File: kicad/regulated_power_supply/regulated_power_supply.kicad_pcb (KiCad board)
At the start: 2 copper layers, 139.1 x 38.5 mm, 43 parts, among them P1 CONN_01X03, P2 CONN_01X02, Q1 Q_NPN_BCE, SW1 SPST, T1 2N3055, U1 TL072, U2 LM723

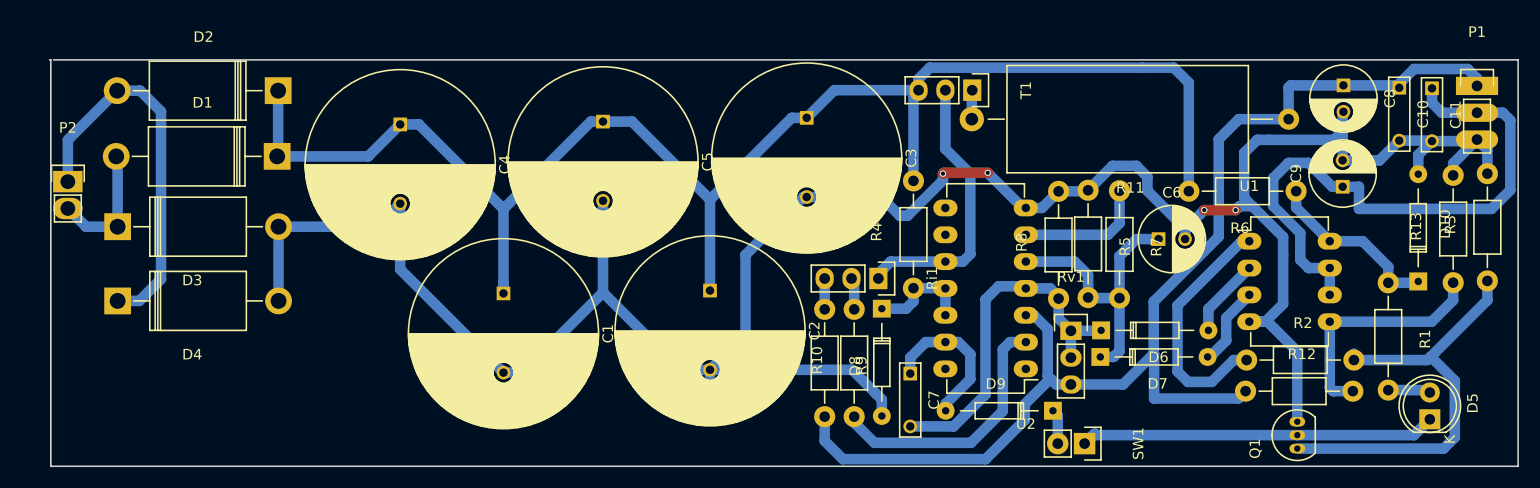
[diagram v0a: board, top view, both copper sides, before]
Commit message: update
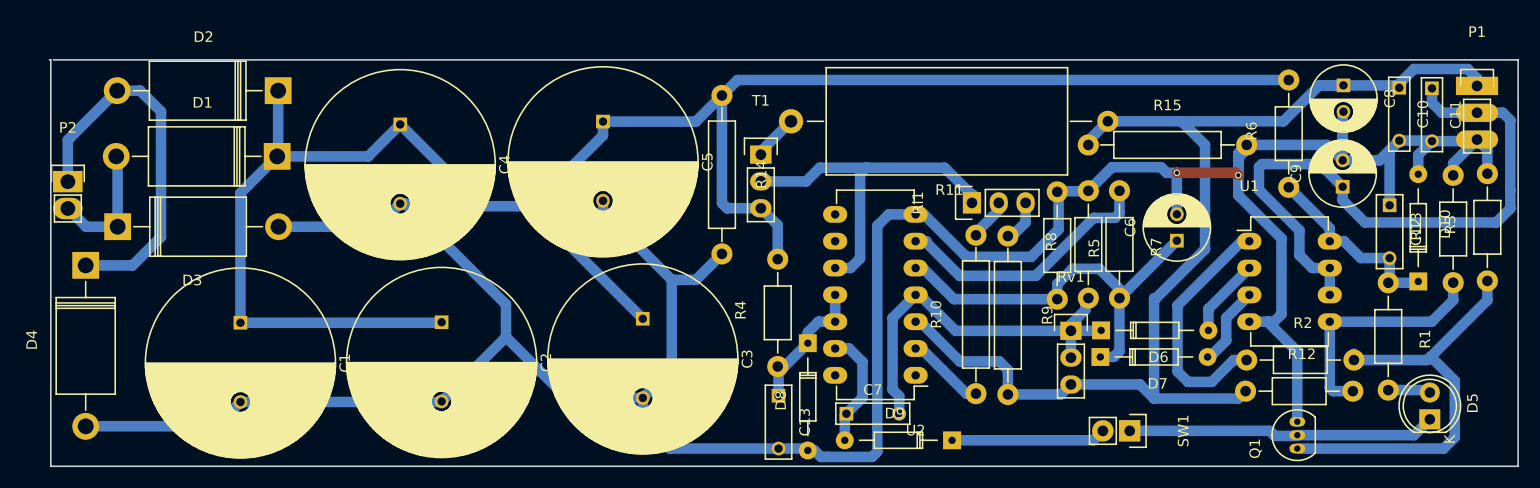
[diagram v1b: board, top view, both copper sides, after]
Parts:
- added C12: 100n, Capacitors_ThroughHole:C_Rect_L7_W2.5_P5, F.Cu at (193.7, 37.3)
- added C13: 100n, Capacitors_ThroughHole:C_Rect_L7_W2.5_P5, F.Cu at (135.8, 55.3)
- added R14: 1K, Resistors_ThroughHole:Resistor_Horizontal_RM15mm, F.Cu at (130.5, 34.4)
- added R15: 1K, Resistors_ThroughHole:Resistor_Horizontal_RM15mm, F.Cu at (172.7, 31.5)
- R10, R9: footprint Resistors_ThroughHole:Resistor_Horizontal_RM10mm -> Resistors_ThroughHole:Resistor_Horizontal_RM15mm
- moved C2 25.6 mm to (103.9, 48.3)
- moved C1 25.1 mm to (84.9, 48.4)
- moved C3 24.6 mm to (123.0, 48.0)
- moved T1 20.9 mm to (134.2, 32.5), turned to 0 degrees
- moved R9 17.9 mm to (157.6, 47.7)
- moved R11 17.1 mm to (152.0, 29.3)
- moved R4 14.8 mm to (135.8, 47.4)
- moved R10 12.4 mm to (154.5, 47.6)
- moved Ri1 11.4 mm to (154.2, 37.0), turned to 90 degrees
- moved U2 10.5 mm to (148.8, 53.4)
- moved D9 9.95 mm to (152.3, 59.5)
- moved D8 7.73 mm to (138.6, 50.3)
- moved C7 7.14 mm to (142.3, 57.0), turned to 0 degrees
- moved R6 6.99 mm to (184.2, 30.5), turned to 90 degrees
- moved D4 4.53 mm to (70.2, 43.0), turned to 270 degrees
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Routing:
- net GND: track 241.3 -> 292.4 mm, vias 4 -> 2
- net /Vin: track 145.9 -> 183.1 mm
- net Net-(R10-Pad1): track 25.7 -> 7.49 mm
- net Net-(R7-Pad1): track 12.4 -> 26.1 mm
- net Net-(C6-Pad1): track 27.1 -> 39.4 mm
- net Net-(D9-Pad1): track 3.30 -> 14.6 mm
- net /Bt1: track 26.4 -> 34.6 mm
- net Net-(D5-Pad1): track 35.0 -> 29.3 mm
- net /Vout: track 115.6 -> 111.1 mm
- net /Vhalf: track 57.4 -> 61.2 mm
- net Net-(C7-Pad1): track 14.6 -> 11.2 mm
- net Net-(C7-Pad2): track 34.4 -> 37.5 mm
- net /V723: track 10.1 -> 13.1 mm
- net Net-(R9-Pad1): track 2.92 -> 4.43 mm
- net Net-(R11-Pad2): track 2.85 -> 4.33 mm
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
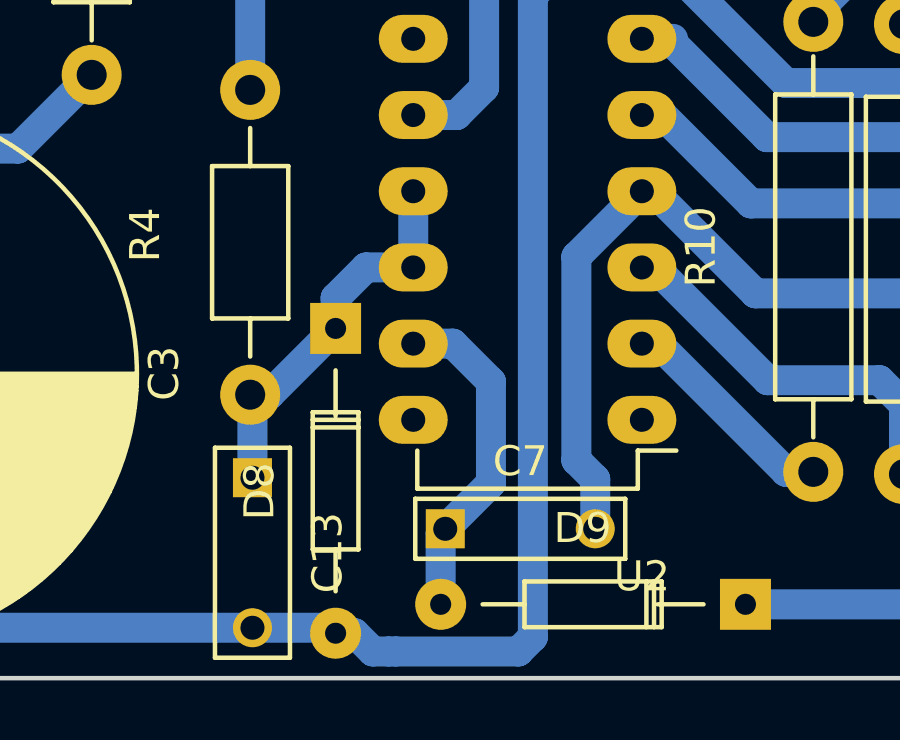
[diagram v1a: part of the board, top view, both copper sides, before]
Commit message: updates
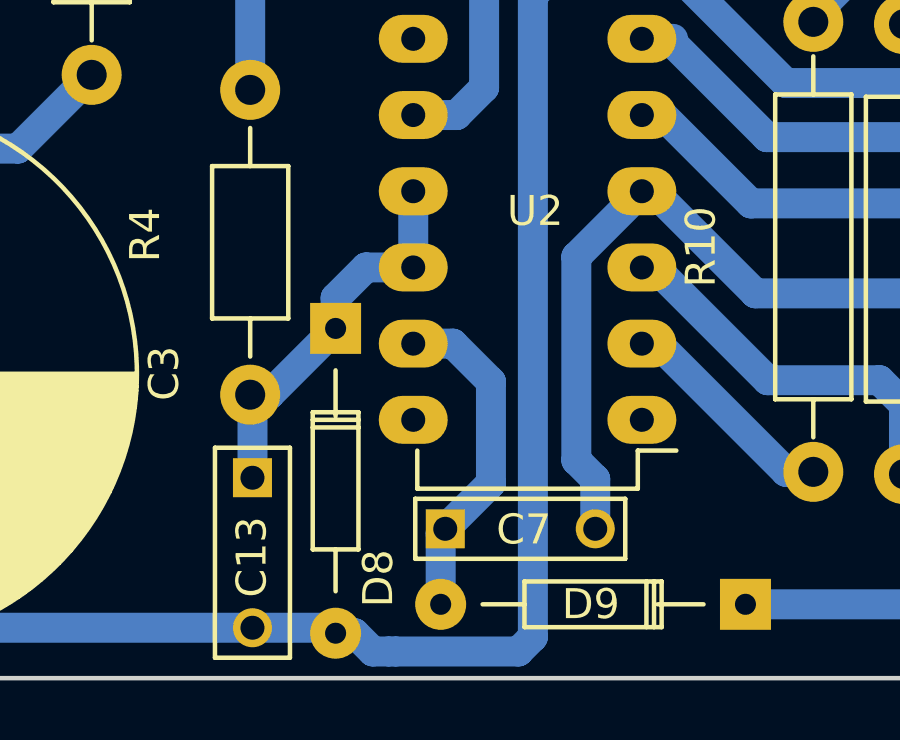
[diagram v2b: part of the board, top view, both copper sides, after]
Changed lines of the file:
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@@
-(kicad_pcb (version 4) (host pcbnew 0.201603161423+6623~43~ubuntu14.04.1-product)
+(kicad_pcb (version 20160815) (host pcbnew 4.1.0-alpha+201608211231+7083~46~ubuntu16.04.1-product)
   (general
     (links 88)
@@
     (uvia_dia 0.3)
     (uvia_drill 0.1)
+    (diff_pair_gap 0.25)
+    (diff_pair_width 0.2)
     (add_net /Bt1)
     (add_net /V723)
@@
     (uvia_dia 0.3)
     (uvia_drill 0.1)
+    (diff_pair_gap 0.25)
+    (diff_pair_width 0.2)
     (add_net /Vin)
     (add_net /Vout)
@@
     (descr "Diode, DO-35,  SOD27, Horizontal, RM 10mm")
     (tags "Diode, DO-35, SOD27, Horizontal, RM 10mm, 1N4148,")
-    (fp_text reference D8 (at 5.43052 2.53746 270) (layer F.SilkS)
-      (effects (font (size 1 1) (thickness 0.15)))
-    )
-    (fp_text value ZENER (at 4.41452 -3.55854 270) (layer F.Fab)
+    (fp_text reference D8 (at 8.3312 -1.4224 270) (layer F.SilkS)
+      (effects (font (size 1 1) (thickness 0.15)))
+    )
+    (fp_text value ZENER (at 5.9436 0.0254 270) (layer F.Fab)
       (effects (font (size 1 1) (thickness 0.15)))
     )
@@
     (descr "14-lead dip package, row spacing 7.62 mm (300 mils), longer pads")
     (tags "dil dip 2.54 300")
-    (fp_text reference U2 (at 0 -5.22 180) (layer F.SilkS)
-      (effects (font (size 1 1) (thickness 0.15)))
-    )
-    (fp_text value LM723 (at 0 -3.72 180) (layer F.Fab)
+    (fp_text reference U2 (at 3.556 6.9596 180) (layer F.SilkS)
+      (effects (font (size 1 1) (thickness 0.15)))
+    )
+    (fp_text value LM723 (at 3.7592 8.763 180) (layer F.Fab)
       (effects (font (size 1 1) (thickness 0.15)))
     )
@@
     (descr "Diode, DO-35,  SOD27, Horizontal, RM 10mm")
     (tags "Diode, DO-35, SOD27, Horizontal, RM 10mm, 1N4148,")
-    (fp_text reference D9 (at 5.43052 2.53746 180) (layer F.SilkS)
-      (effects (font (size 1 1) (thickness 0.15)))
-    )
-    (fp_text value 1n4148 (at 4.41452 -3.55854 180) (layer F.Fab)
+    (fp_text reference D9 (at 5.1562 0 180) (layer F.SilkS)
+      (effects (font (size 1 1) (thickness 0.15)))
+    )
+    (fp_text value 1n4148 (at 6.0452 -1.6002 180) (layer F.Fab)
       (effects (font (size 1 1) (thickness 0.15)))
     )
@@
     (descr "Film Capacitor Length 7 x Width 2mm, Pitch 5mm")
     (tags Capacitor)
-    (fp_text reference C7 (at 2.5 -2.25) (layer F.SilkS)
-      (effects (font (size 1 1) (thickness 0.15)))
-    )
-    (fp_text value 470 (at 2.5 2.5) (layer F.Fab)
+    (fp_text reference C7 (at 2.6162 0.0254) (layer F.SilkS)
+      (effects (font (size 1 1) (thickness 0.15)))
+    )
+    (fp_text value 470 (at 7.8486 0.2032) (layer F.Fab)
       (effects (font (size 1 1) (thickness 0.15)))
     )
@@
     (descr "Film Capacitor Length 7mm x Width 2.5mm, Pitch 5mm")
     (tags Capacitor)
-    (fp_text reference C13 (at 2.5 -2.5 270) (layer F.SilkS)
-      (effects (font (size 1 1) (thickness 0.15)))
-    )
+    (fp_text reference C13 (at 2.6416 0.0254 270) (layer F.SilkS)
+      (effects (font (size 1 1) (thickness 0.15)))
+    )
